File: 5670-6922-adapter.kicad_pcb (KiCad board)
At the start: 2 copper layers, 23 x 23 mm, 2 parts, among them J1 5670-Socket, J2 6922-Pins

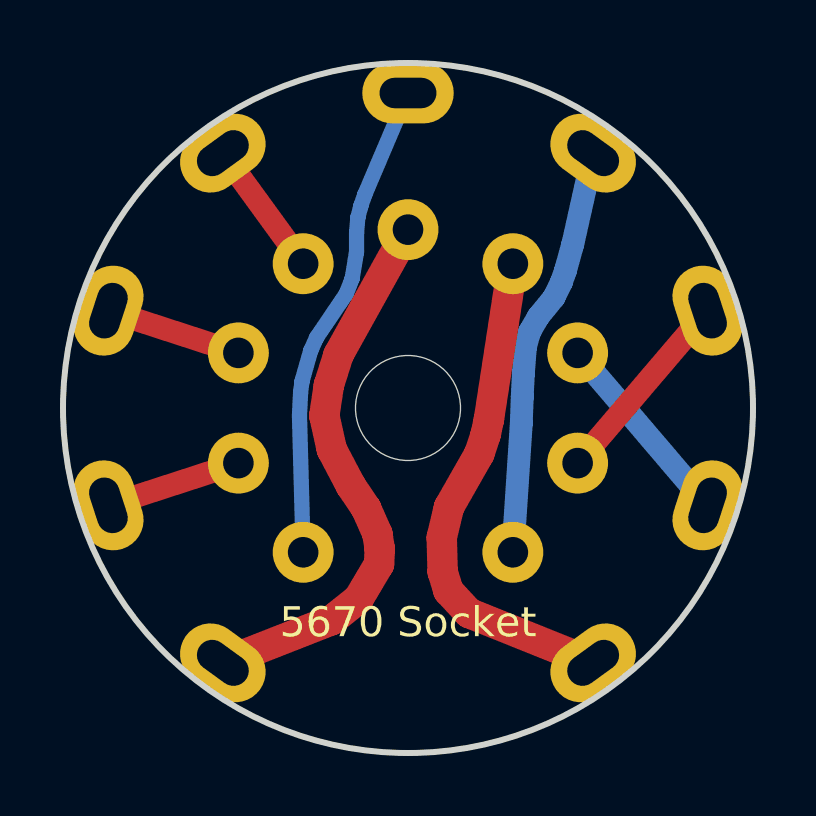
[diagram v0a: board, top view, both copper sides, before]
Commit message: Publish final PCB
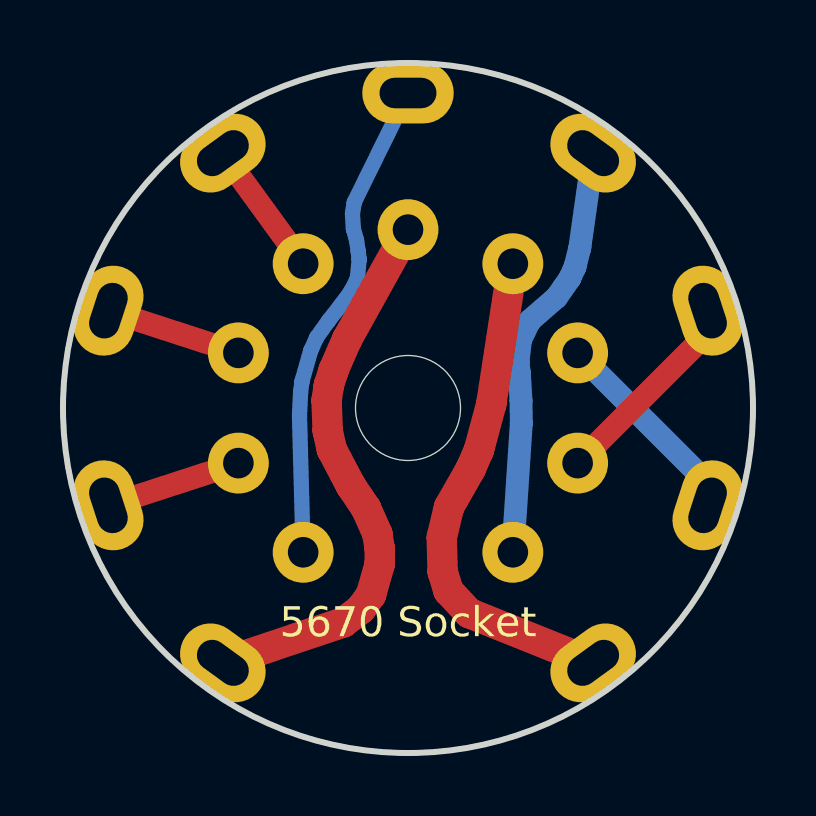
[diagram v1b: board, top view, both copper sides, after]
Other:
- net class Default: trace_width 0.508 -> 1.016
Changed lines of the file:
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@@
     (thickness 1.6)
     (drawings 4)
-    (tracks 50)
+    (tracks 58)
     (zones 0)
     (modules 2)
@@
   )
   (setup
-    (last_trace_width 0.508)
+    (last_trace_width 1.016)
     (trace_clearance 0.254)
     (zone_clearance 0.508)
@@
     (solder_mask_min_width 0.25)
     (aux_axis_origin 0 0)
-    (visible_elements FFFFFF7F)
+    (visible_elements 7FFFFFFF)
     (pcbplotparams
       (layerselection 0x010f0_ffffffff)
@@
   (net_class Default "This is the default net class."
     (clearance 0.254)
-    (trace_width 0.508)
+    (trace_width 1.016)
     (via_dia 0.8)
     (via_drill 0.4)
@@
   (gr_circle (center 95.25 79.375) (end 98.5 79.375) (layer B.SilkS) (width 0.2))
   (gr_circle (center 95.25 79.375) (end 106.75 79.375) (layer Edge.Cuts) (width 0.2))
-  (segment (start 92.933994 77.597) (end 95.25 73.43) (width 1.016) (layer F.Cu) (net 1))
-  (segment (start 92.460355 79.629) (end 92.71 80.756592) (width 1.016) (layer F.Cu) (net 1))
-  (segment (start 93.599 85.7377) (end 94.2848 84.582) (width 1.016) (layer F.Cu) (net 1))
-  (segment (start 93.599 85.7377) (end 92.71 86.444047) (width 1.016) (layer F.Cu) (net 1))
-  (segment (start 89.078255 87.869678) (end 92.71 86.444047) (width 1.016) (layer F.Cu) (net 1))
   (segment (start 92.71 80.756592) (end 93.345 81.966085) (width 1.016) (layer F.Cu) (net 1))
-  (segment (start 92.460355 79.629) (end 92.612172 78.613) (width 1.016) (layer F.Cu) (net 1))
-  (segment (start 92.933994 77.597) (end 92.612172 78.613) (width 1.016) (layer F.Cu) (net 1))
-  (segment (start 94.3102 84.074) (end 94.2848 84.582) (width 1.016) (layer F.Cu) (net 1))
   (segment (start 93.853 82.718583) (end 94.228869 83.566) (width 1.016) (layer F.Cu) (net 1))
   (segment (start 94.228869 83.566) (end 94.3102 84.074) (width 1.016) (layer F.Cu) (net 1))
   (segment (start 93.345 81.966085) (end 93.853 82.718583) (width 1.016) (layer F.Cu) (net 1))
+  (segment (start 92.572825 80.137) (end 92.536264 79.121) (width 1.016) (layer F.Cu) (net 1))
+  (segment (start 92.536264 79.121) (end 92.612172 78.613) (width 1.016) (layer F.Cu) (net 1))
+  (segment (start 92.572825 80.137) (end 92.71 80.756592) (width 1.016) (layer F.Cu) (net 1))
+  (segment (start 93.216339 77.089) (end 92.773083 78.105) (width 1.016) (layer F.Cu) (net 1))
+  (segment (start 92.773083 78.105) (end 92.612172 78.613) (width 1.016) (layer F.Cu) (net 1))
+  (segment (start 93.216339 77.089) (end 95.25 73.43) (width 1.016) (layer F.Cu) (net 1))
+  (segment (start 94.3102 84.074) (end 94.306465 84.582) (width 1.016) (layer F.Cu) (net 1))
+  (segment (start 93.091 86.524291) (end 89.078255 87.869678) (width 1.016) (layer F.Cu) (net 1))
+  (segment (start 94.019216 85.598) (end 94.306465 84.582) (width 1.016) (layer F.Cu) (net 1))
+  (segment (start 94.019216 85.598) (end 93.6752 86.079115) (width 1.016) (layer F.Cu) (net 1))
+  (segment (start 93.6752 86.079115) (end 93.091 86.524291) (width 1.016) (layer F.Cu) (net 1))
   (segment (start 89.595969 81.212106) (end 85.263907 82.619678) (width 0.762) (layer F.Cu) (net 2))
   (segment (start 89.595969 77.537894) (end 85.263907 76.130322) (width 0.762) (layer F.Cu) (net 3))
@@
   (segment (start 91.716173 78.486) (end 92.00501 77.47) (width 0.508) (layer B.Cu) (net 5))
   (segment (start 92.00501 77.47) (end 92.202 77.027313) (width 0.508) (layer B.Cu) (net 5))
-  (segment (start 92.202 77.027313) (end 93.192709 75.565) (width 0.508) (layer B.Cu) (net 5))
-  (segment (start 93.5355 74.168) (end 93.38859 75.057) (width 0.508) (layer B.Cu) (net 5))
-  (segment (start 93.38859 75.057) (end 93.192709 75.565) (width 0.508) (layer B.Cu) (net 5))
-  (segment (start 93.577991 73.025) (end 93.5355 73.533) (width 0.508) (layer B.Cu) (net 5))
-  (segment (start 93.5355 74.168) (end 93.5355 73.533) (width 0.508) (layer B.Cu) (net 5))
   (segment (start 91.669086 78.867) (end 91.632312 79.629) (width 0.508) (layer B.Cu) (net 5))
   (segment (start 91.755617 84.184606) (end 91.632312 79.629) (width 0.508) (layer B.Cu) (net 5))
   (segment (start 91.669086 78.867) (end 91.716173 78.486) (width 0.508) (layer B.Cu) (net 5))
-  (segment (start 93.577991 73.025) (end 93.677243 72.644) (width 0.508) (layer B.Cu) (net 5))
-  (segment (start 93.808459 72.263) (end 95.25 68.875) (width 0.508) (layer B.Cu) (net 5))
-  (segment (start 93.677243 72.644) (end 93.808459 72.263) (width 0.508) (layer B.Cu) (net 5))
+  (segment (start 93.5355 73.787) (end 93.59265 74.168) (width 0.508) (layer B.Cu) (net 5))
+  (segment (start 93.398488 72.898) (end 93.429666 73.406) (width 0.508) (layer B.Cu) (net 5))
+  (segment (start 93.5355 73.787) (end 93.429666 73.406) (width 0.508) (layer B.Cu) (net 5))
+  (segment (start 93.398488 72.898) (end 93.457555 72.517) (width 0.508) (layer B.Cu) (net 5))
+  (segment (start 93.457555 72.517) (end 95.25 68.875) (width 0.508) (layer B.Cu) (net 5))
+  (segment (start 93.561958 75.057) (end 93.622283 74.422) (width 0.508) (layer B.Cu) (net 5))
+  (segment (start 93.59265 74.168) (end 93.622283 74.422) (width 0.508) (layer B.Cu) (net 5))
+  (segment (start 93.010181 75.946) (end 92.610675 76.454) (width 0.508) (layer B.Cu) (net 5))
+  (segment (start 92.202 77.027313) (end 92.610675 76.454) (width 0.508) (layer B.Cu) (net 5))
+  (segment (start 93.010181 75.946) (end 93.345 75.486361) (width 0.508) (layer B.Cu) (net 5))
+  (segment (start 93.561958 75.057) (end 93.345 75.486361) (width 0.508) (layer B.Cu) (net 5))
   (segment (start 98.744383 84.184606) (end 99.026664 79.883) (width 0.762) (layer B.Cu) (net 6))
-  (segment (start 100.114841 75.692) (end 99.597494 76.327) (width 0.762) (layer B.Cu) (net 6))
-  (segment (start 99.597494 76.327) (end 99.30435 76.835) (width 0.762) (layer B.Cu) (net 6))
-  (segment (start 99.30435 76.835) (end 99.16286 77.343) (width 0.762) (layer B.Cu) (net 6))
-  (segment (start 99.095347 78.232) (end 99.16286 77.343) (width 0.762) (layer B.Cu) (net 6))
-  (segment (start 99.058741 78.994) (end 99.026664 79.883) (width 0.762) (layer B.Cu) (net 6))
-  (segment (start 99.095347 78.232) (end 99.058741 78.994) (width 0.762) (layer B.Cu) (net 6))
-  (segment (start 100.114841 75.692) (end 100.3633 75.184) (width 0.762) (layer B.Cu) (net 6))
-  (segment (start 100.3633 75.184) (end 100.496473 74.803) (width 0.762) (layer B.Cu) (net 6))
-  (segment (start 100.742793 73.914) (end 101.421745 70.880322) (width 0.762) (layer B.Cu) (net 6))
-  (segment (start 100.496473 74.803) (end 100.742793 73.914) (width 0.762) (layer B.Cu) (net 6))
-  (segment (start 100.904031 81.212106) (end 105.236093 76.130322) (width 0.762) (layer F.Cu) (net 7))
-  (segment (start 105.236093 82.619678) (end 100.904031 77.537894) (width 0.762) (layer B.Cu) (net 8))
-  (segment (start 98.744383 74.565394) (end 97.947029 79.756) (width 1.016) (layer F.Cu) (net 9))
+  (segment (start 100.976853 74.041) (end 101.421745 70.880322) (width 0.762) (layer B.Cu) (net 6))
+  (segment (start 100.816065 74.676) (end 100.976853 74.041) (width 0.762) (layer B.Cu) (net 6))
+  (segment (start 100.642809 75.057) (end 100.203 75.686478) (width 0.762) (layer B.Cu) (net 6))
+  (segment (start 100.642809 75.057) (end 100.816065 74.676) (width 0.762) (layer B.Cu) (net 6))
+  (segment (start 99.00318 77.089) (end 99.314 76.459521) (width 0.762) (layer B.Cu) (net 6))
+  (segment (start 100.203 75.686478) (end 99.314 76.459521) (width 0.762) (layer B.Cu) (net 6))
+  (segment (start 99.00318 77.089) (end 98.915872 77.851) (width 0.762) (layer B.Cu) (net 6))
+  (segment (start 98.963495 78.232) (end 99.017337 79.121) (width 0.762) (layer B.Cu) (net 6))
+  (segment (start 99.017337 79.121) (end 99.026664 79.883) (width 0.762) (layer B.Cu) (net 6))
+  (segment (start 98.915872 77.851) (end 98.963495 78.232) (width 0.762) (layer B.Cu) (net 6))
+  (segment (start 105.236093 76.880044) (end 100.904031 81.212106) (width 0.762) (layer F.Cu) (net 7))
+  (segment (start 105.236093 76.130322) (end 105.236093 76.880044) (width 0.762) (layer F.Cu) (net 7))
+  (segment (start 105.236093 81.869956) (end 100.904031 77.537894) (width 0.762) (layer B.Cu) (net 8))
+  (segment (start 105.236093 82.619678) (end 105.236093 81.869956) (width 0.762) (layer B.Cu) (net 8))
   (segment (start 97.282 86.208694) (end 101.421745 87.869678) (width 1.016) (layer F.Cu) (net 9))
   (segment (start 97.282 86.208694) (end 96.598853 85.471) (width 1.016) (layer F.Cu) (net 9))
-  (segment (start 97.947029 79.756) (end 97.837036 80.264) (width 1.016) (layer F.Cu) (net 9))
-  (segment (start 97.628616 80.899) (end 97.837036 80.264) (width 1.016) (layer F.Cu) (net 9))
   (segment (start 96.405115 84.836) (end 96.598853 85.471) (width 1.016) (layer F.Cu) (net 9))
   (segment (start 96.374419 83.693) (end 96.405115 84.836) (width 1.016) (layer F.Cu) (net 9))
   (segment (start 96.374419 83.693) (end 96.61665 82.677) (width 1.016) (layer F.Cu) (net 9))
-  (segment (start 97.628616 80.899) (end 96.61665 82.677) (width 1.016) (layer F.Cu) (net 9))
+  (segment (start 97.339482 81.407) (end 96.61665 82.677) (width 1.016) (layer F.Cu) (net 9))
+  (segment (start 97.339482 81.407) (end 97.615901 80.772) (width 1.016) (layer F.Cu) (net 9))
+  (segment (start 97.615901 80.772) (end 98.025066 79.248) (width 1.016) (layer F.Cu) (net 9))
+  (segment (start 98.744383 74.565394) (end 98.025066 79.248) (width 1.016) (layer F.Cu) (net 9))
 )
